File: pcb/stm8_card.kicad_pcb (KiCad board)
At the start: 2 copper layers, 101.9 x 50.9 mm, 22 parts, among them J1 DEBUG HEADER, SW1 TL59AF100Q, SW2 TL59AF100Q, SW3 TL59AF100Q, SW4 TL3302AF260QG, U1 ER-OLED0.91-7, U2 STM8S103F3

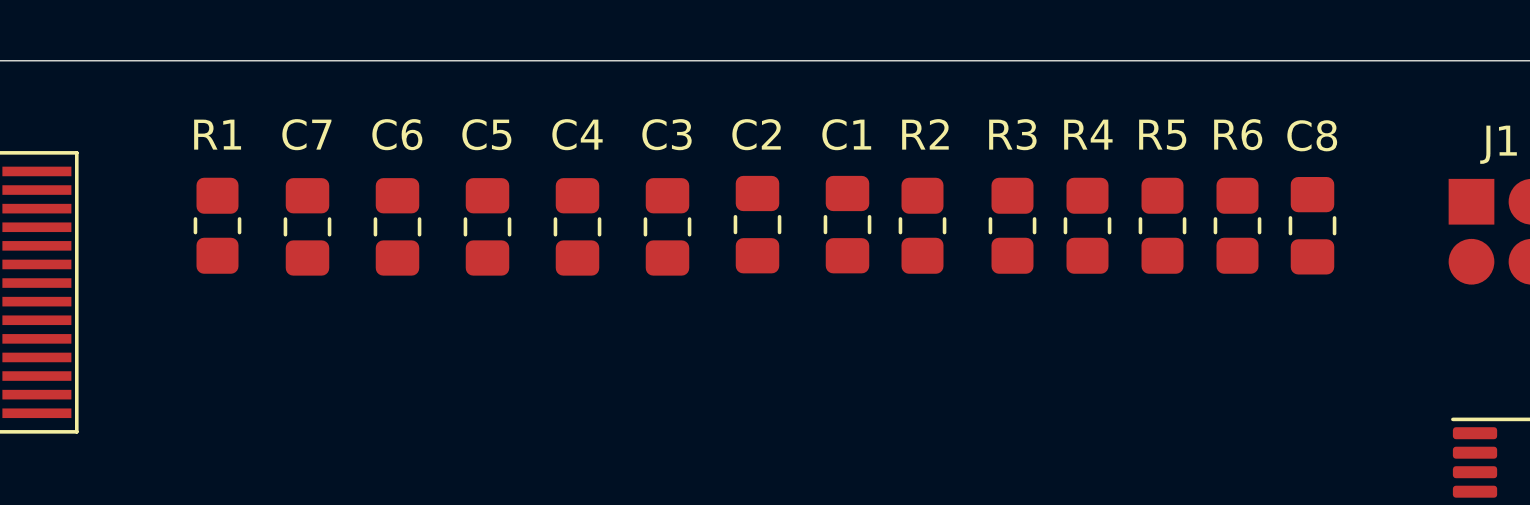
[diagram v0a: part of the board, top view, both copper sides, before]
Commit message: pcb small edits
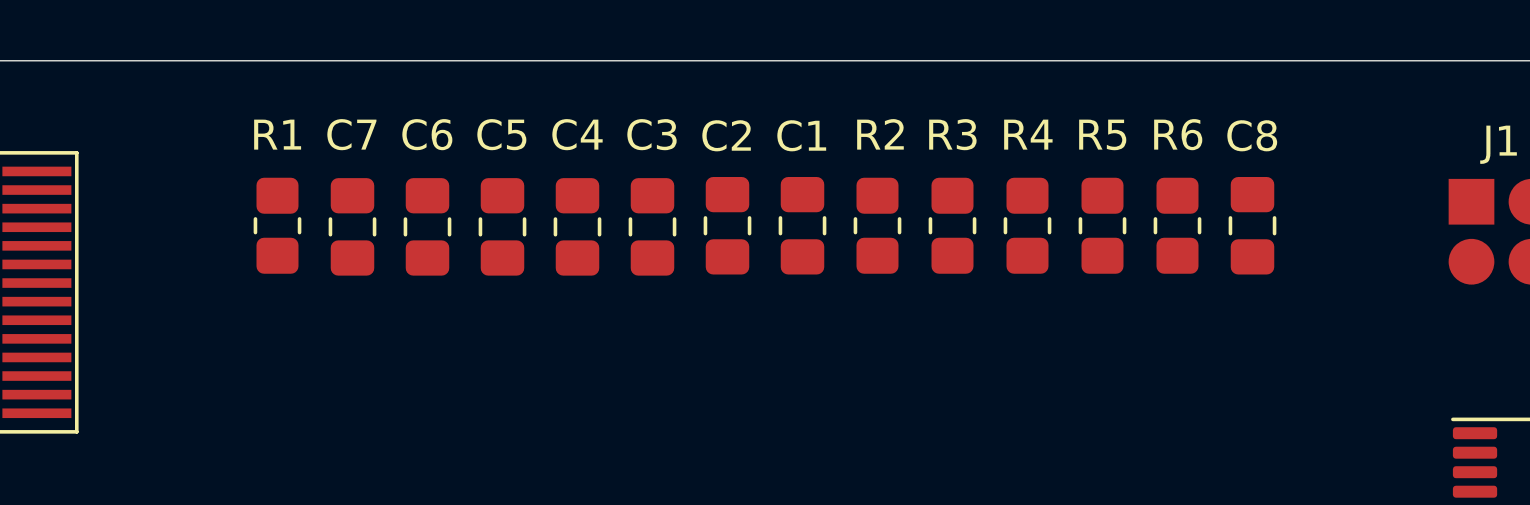
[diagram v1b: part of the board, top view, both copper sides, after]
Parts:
- moved C8 2.00 mm to (261.5, 107.0)
- moved R1 2.00 mm to (229.0, 107.0)
- moved R3 2.00 mm to (251.5, 107.0)
- moved R4 2.00 mm to (254.0, 107.0), turned to 270 degrees
- moved R5 2.00 mm to (256.5, 107.0)
- moved R6 2.00 mm to (259.0, 107.0)
- moved C1 1.50 mm to (246.5, 107.0)
- moved C7 1.50 mm to (231.5, 107.0)
- moved R2 1.50 mm to (249.0, 107.0)
- moved C2 1.00 mm to (244.0, 107.0)
- moved C6 1.00 mm to (234.0, 107.0)
- moved C3 0.50 mm to (241.5, 107.0)
- moved C5 0.50 mm to (236.5, 107.0)
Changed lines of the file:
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@@
   )
   (module Capacitor_SMD:C_0805_2012Metric_Pad1.18x1.45mm_HandSolder (layer F.Cu)
-    (at 248 106.9625 90)
+    (at 246.5 107 90)
     (descr "Capacitor SMD 0805 (2012 Metric), square (rectangular) end terminal, IPC_7351 nominal with elongated pad for handsoldering. (Body size source: IPC-SM-782 page 76, https://www.pcb-3d.com/wordpress/wp-content/uploads/ipc-sm-782a_amendment_1_and_2.pdf, https://docs.google.com/spreadsheets/d/1BsfQQcO9C6DZCsRaXUlFlo91Tg2WpOkGARC1WS5S8t0/edit?usp=sharing), generated with kicad-footprint-generator")
     (tags "capacitor handsolder")
@@
   )
   (module Capacitor_SMD:C_0805_2012Metric_Pad1.18x1.45mm_HandSolder (layer F.Cu)
-    (at 245 106.9625 90)
+    (at 244 107 90)
     (descr "Capacitor SMD 0805 (2012 Metric), square (rectangular) end terminal, IPC_7351 nominal with elongated pad for handsoldering. (Body size source: IPC-SM-782 page 76, https://www.pcb-3d.com/wordpress/wp-content/uploads/ipc-sm-782a_amendment_1_and_2.pdf, https://docs.google.com/spreadsheets/d/1BsfQQcO9C6DZCsRaXUlFlo91Tg2WpOkGARC1WS5S8t0/edit?usp=sharing), generated with kicad-footprint-generator")
     (tags "capacitor handsolder")
@@
   )
   (module Capacitor_SMD:C_0805_2012Metric_Pad1.18x1.45mm_HandSolder (layer F.Cu)
-    (at 242 107.0375 90)
+    (at 241.5 107.0375 90)
     (descr "Capacitor SMD 0805 (2012 Metric), square (rectangular) end terminal, IPC_7351 nominal with elongated pad for handsoldering. (Body size source: IPC-SM-782 page 76, https://www.pcb-3d.com/wordpress/wp-content/uploads/ipc-sm-782a_amendment_1_and_2.pdf, https://docs.google.com/spreadsheets/d/1BsfQQcO9C6DZCsRaXUlFlo91Tg2WpOkGARC1WS5S8t0/edit?usp=sharing), generated with kicad-footprint-generator")
     (tags "capacitor handsolder")
@@
   )
   (module Capacitor_SMD:C_0805_2012Metric_Pad1.18x1.45mm_HandSolder (layer F.Cu)
-    (at 236 107.0375 270)
+    (at 236.5 107.0375 270)
     (descr "Capacitor SMD 0805 (2012 Metric), square (rectangular) end terminal, IPC_7351 nominal with elongated pad for handsoldering. (Body size source: IPC-SM-782 page 76, https://www.pcb-3d.com/wordpress/wp-content/uploads/ipc-sm-782a_amendment_1_and_2.pdf, https://docs.google.com/spreadsheets/d/1BsfQQcO9C6DZCsRaXUlFlo91Tg2WpOkGARC1WS5S8t0/edit?usp=sharing), generated with kicad-footprint-generator")
     (tags "capacitor handsolder")
@@
   )
   (module Capacitor_SMD:C_0805_2012Metric_Pad1.18x1.45mm_HandSolder (layer F.Cu)
-    (at 233 107.0375 270)
+    (at 234 107.0375 270)
     (descr "Capacitor SMD 0805 (2012 Metric), square (rectangular) end terminal, IPC_7351 nominal with elongated pad for handsoldering. (Body size source: IPC-SM-782 page 76, https://www.pcb-3d.com/wordpress/wp-content/uploads/ipc-sm-782a_amendment_1_and_2.pdf, https://docs.google.com/spreadsheets/d/1BsfQQcO9C6DZCsRaXUlFlo91Tg2WpOkGARC1WS5S8t0/edit?usp=sharing), generated with kicad-footprint-generator")
     (tags "capacitor handsolder")
@@
   )
   (module Capacitor_SMD:C_0805_2012Metric_Pad1.18x1.45mm_HandSolder (layer F.Cu)
-    (at 230 107.0375 270)
+    (at 231.5 107.0375 270)
     (descr "Capacitor SMD 0805 (2012 Metric), square (rectangular) end terminal, IPC_7351 nominal with elongated pad for handsoldering. (Body size source: IPC-SM-782 page 76, https://www.pcb-3d.com/wordpress/wp-content/uploads/ipc-sm-782a_amendment_1_and_2.pdf, https://docs.google.com/spreadsheets/d/1BsfQQcO9C6DZCsRaXUlFlo91Tg2WpOkGARC1WS5S8t0/edit?usp=sharing), generated with kicad-footprint-generator")
     (tags "capacitor handsolder")
@@
   )
   (module Capacitor_SMD:C_0805_2012Metric_Pad1.18x1.45mm_HandSolder (layer F.Cu)
-    (at 263.5 107 90)
+    (at 261.5 107 90)
     (descr "Capacitor SMD 0805 (2012 Metric), square (rectangular) end terminal, IPC_7351 nominal with elongated pad for handsoldering. (Body size source: IPC-SM-782 page 76, https://www.pcb-3d.com/wordpress/wp-content/uploads/ipc-sm-782a_amendment_1_and_2.pdf, https://docs.google.com/spreadsheets/d/1BsfQQcO9C6DZCsRaXUlFlo91Tg2WpOkGARC1WS5S8t0/edit?usp=sharing), generated with kicad-footprint-generator")
     (tags "capacitor handsolder")
@@
   )
   (module Resistor_SMD:R_0805_2012Metric_Pad1.20x1.40mm_HandSolder (layer F.Cu)
-    (at 227 107 90)
+    (at 229 107 90)
     (descr "Resistor SMD 0805 (2012 Metric), square (rectangular) end terminal, IPC_7351 nominal with elongated pad for handsoldering. (Body size source: IPC-SM-782 page 72, https://www.pcb-3d.com/wordpress/wp-content/uploads/ipc-sm-782a_amendment_1_and_2.pdf), generated with kicad-footprint-generator")
     (tags "resistor handsolder")
@@
   )
   (module Resistor_SMD:R_0805_2012Metric_Pad1.20x1.40mm_HandSolder (layer F.Cu)
-    (at 250.5 107 90)
+    (at 249 107 90)
     (descr "Resistor SMD 0805 (2012 Metric), square (rectangular) end terminal, IPC_7351 nominal with elongated pad for handsoldering. (Body size source: IPC-SM-782 page 72, https://www.pcb-3d.com/wordpress/wp-content/uploads/ipc-sm-782a_amendment_1_and_2.pdf), generated with kicad-footprint-generator")
     (tags "resistor handsolder")
@@
   )
   (module Resistor_SMD:R_0805_2012Metric_Pad1.20x1.40mm_HandSolder (layer F.Cu)
-    (at 253.5 107 90)
+    (at 251.5 107 90)
     (descr "Resistor SMD 0805 (2012 Metric), square (rectangular) end terminal, IPC_7351 nominal with elongated pad for handsoldering. (Body size source: IPC-SM-782 page 72, https://www.pcb-3d.com/wordpress/wp-content/uploads/ipc-sm-782a_amendment_1_and_2.pdf), generated with kicad-footprint-generator")
     (tags "resistor handsolder")
@@
   )
   (module Resistor_SMD:R_0805_2012Metric_Pad1.20x1.40mm_HandSolder (layer F.Cu)
-    (at 256 107 90)
-    (descr "Resistor SMD 0805 (2012 Metric), square (rectangular) end terminal, IPC_7351 nominal with elongated pad for handsoldering. (Body size source: IPC-SM-782 page 72, https://www.pcb-3d.com/wordpress/wp-content/uploads/ipc-sm-782a_amendment_1_and_2.pdf), generated with kicad-footprint-generator")
-    (tags "resistor handsolder")
-    (attr smd)
-    (fp_text reference R4 (at 3 0 180) (layer F.SilkS)
+    (at 254 107 270)
+    (descr "Resistor SMD 0805 (2012 Metric), square (rectangular) end terminal, IPC_7351 nominal with elongated pad for handsoldering. (Body size source: IPC-SM-782 page 72, https://www.pcb-3d.com/wordpress/wp-content/uploads/ipc-sm-782a_amendment_1_and_2.pdf), generated with kicad-footprint-generator")
+    (tags "resistor handsolder")
+    (attr smd)
+    (fp_text reference R4 (at -3 0 180) (layer F.SilkS)
       (effects (font (size 1 1) (thickness 0.15)))
     )
@@
       (effects (font (size 0.5 0.5) (thickness 0.08)))
     )
-    (pad 1 smd roundrect (at -1 0 90) (size 1.2 1.4) (layers F.Cu F.Paste F.Mask) (roundrect_rratio 0.208333)
-      (net 1 GND))
-    (pad 2 smd roundrect (at 1 0 90) (size 1.2 1.4) (layers F.Cu F.Paste F.Mask) (roundrect_rratio 0.208333)
+    (pad 1 smd roundrect (at -1 0 270) (size 1.2 1.4) (layers F.Cu F.Paste F.Mask) (roundrect_rratio 0.208333)
+      (net 1 GND))
+    (pad 2 smd roundrect (at 1 0 270) (size 1.2 1.4) (layers F.Cu F.Paste F.Mask) (roundrect_rratio 0.208333)
       (net 20 btn0))
     (model ${KISYS3DMOD}/Resistor_SMD.3dshapes/R_0805_2012Metric.wrl
@@
   )
   (module Resistor_SMD:R_0805_2012Metric_Pad1.20x1.40mm_HandSolder (layer F.Cu)
-    (at 258.5 107 270)
+    (at 256.5 107 270)
     (descr "Resistor SMD 0805 (2012 Metric), square (rectangular) end terminal, IPC_7351 nominal with elongated pad for handsoldering. (Body size source: IPC-SM-782 page 72, https://www.pcb-3d.com/wordpress/wp-content/uploads/ipc-sm-782a_amendment_1_and_2.pdf), generated with kicad-footprint-generator")
     (tags "resistor handsolder")
@@
   )
   (module Resistor_SMD:R_0805_2012Metric_Pad1.20x1.40mm_HandSolder (layer F.Cu)
-    (at 261 107 270)
-    (descr "Resistor SMD 0805 (2012 Metric), square (rectangular) end terminal, IPC_7351 nominal with elongated pad for handsoldering. (Body size source: IPC-SM-782 page 72, https://www.pcb-3d.com/wordpress/wp-content/uploads/ipc-sm-782a_amendment_1_and_2.pdf), generated with kicad-footprint-generator")
-    (tags "resistor handsolder")
+    (at 259 107 270)
+    (descr "Resistor SMD 0805 (2012 Metric), square (rectangular) end terminal, IPC_7351 nominal with elongated pad for handsoldering. (Body size source: IPC-SM-782 page 72, https://www.pcb-3d.com/wordpress/wp-content/uploads/ipc-sm-782a_amendment_1_and_2.pdf), generated with kicad-footprint-generator")
+    (tags "resistor handsolder")

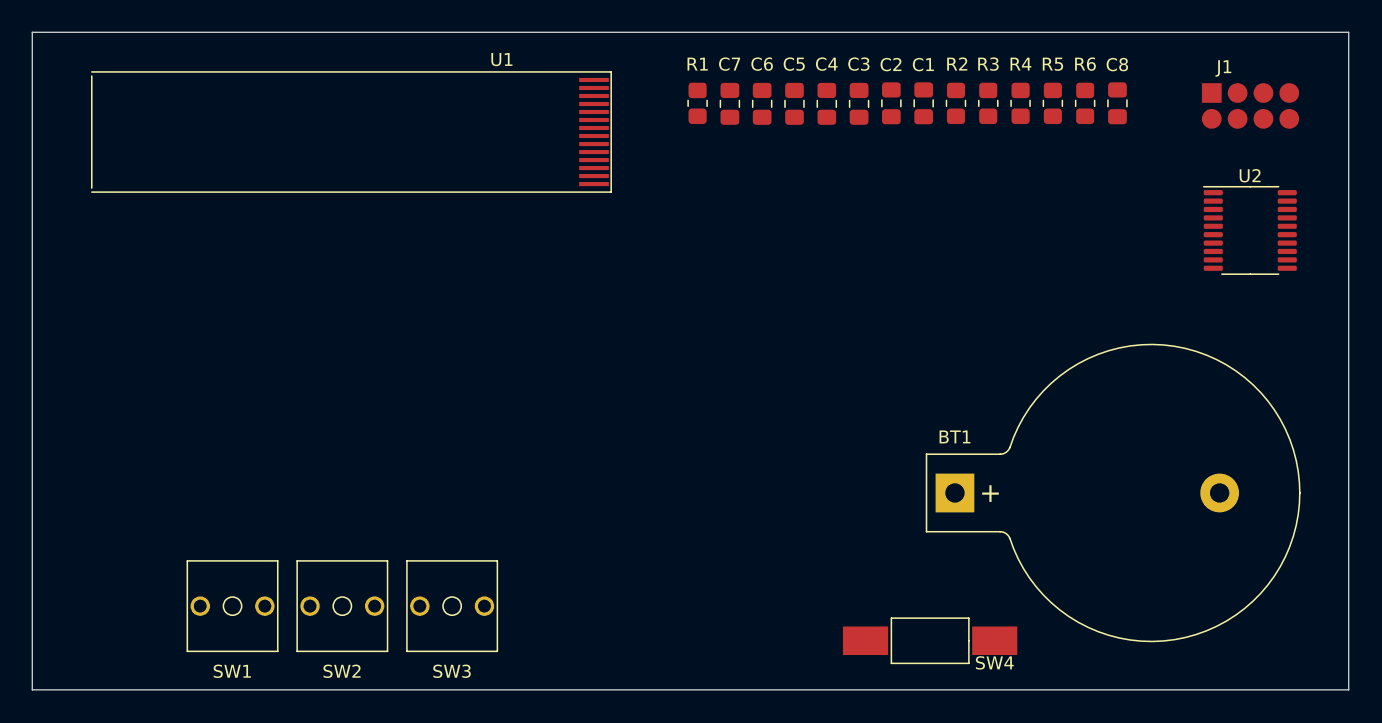
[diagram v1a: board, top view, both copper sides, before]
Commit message: pcb technically finished I think?
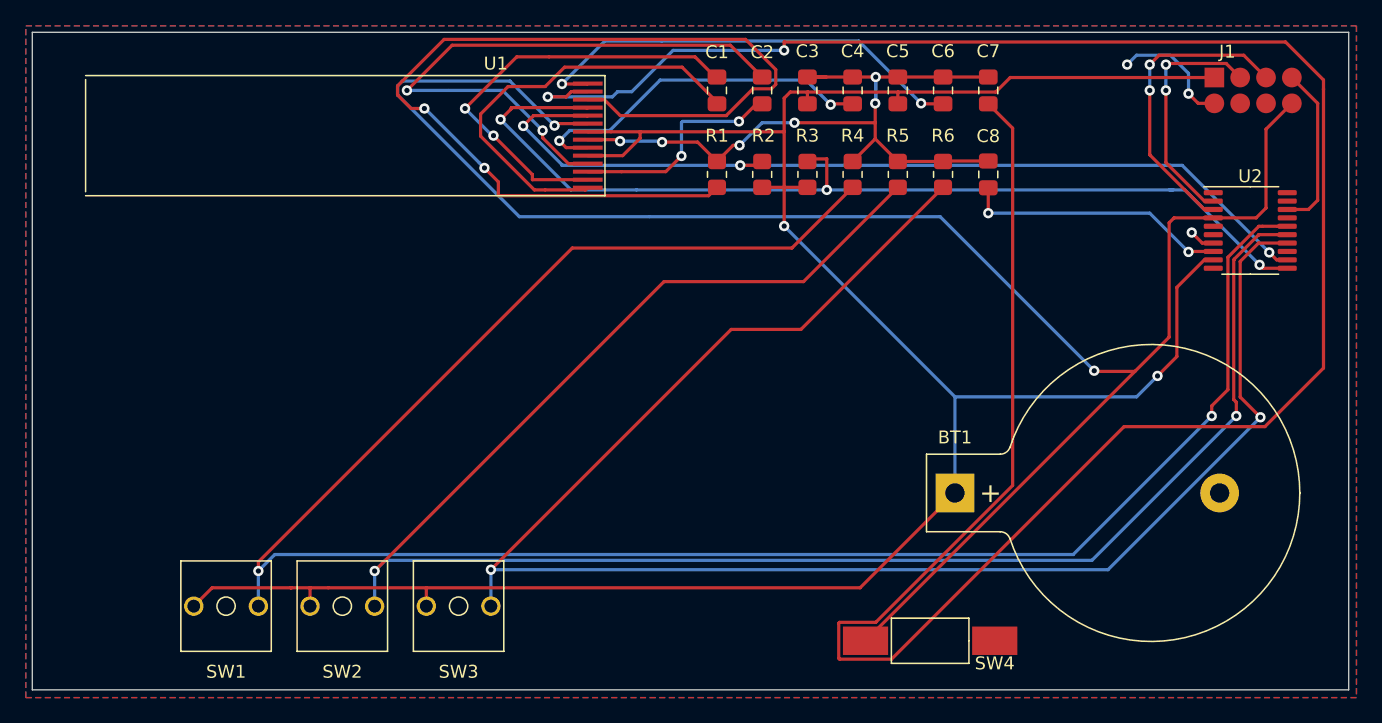
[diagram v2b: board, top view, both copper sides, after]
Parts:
- moved C7 20.0 mm to (251.5, 106.0)
- moved C1 16.0 mm to (230.5, 106.0)
- moved R2 16.0 mm to (234.0, 112.5)
- moved R3 15.0 mm to (237.5, 112.5)
- moved R4 14.1 mm to (241.0, 112.5)
- moved C6 14.0 mm to (248.0, 106.0)
- moved R5 13.2 mm to (244.5, 112.5)
- moved R6 12.3 mm to (248.0, 112.5)
- moved C8 11.4 mm to (251.5, 112.5)
- moved C2 10.0 mm to (234.0, 106.0)
- moved C5 8.07 mm to (244.5, 106.0)
- moved R1 5.70 mm to (230.5, 112.5)
- moved C3 4.13 mm to (237.5, 106.0)
- moved C4 2.25 mm to (241.0, 106.0)
- moved J1 1.22 mm to (272.0, 106.0)
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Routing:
- net 3v3: track 0.00 -> 188.7 mm, vias 0 -> 2
- net Net-(C7-Pad2): track 0.00 -> 186.9 mm, vias 0 -> 2
- net btn0: track 0.00 -> 159.3 mm, vias 0 -> 2
- net btn1: track 0.00 -> 145.0 mm, vias 0 -> 2
- net NRST: track 0.00 -> 142.7 mm, vias 0 -> 2
- net btn2: track 0.00 -> 131.5 mm, vias 0 -> 2
- net Net-(R1-Pad1): track 0.00 -> 78.5 mm, vias 0 -> 2
- net SDA: track 0.00 -> 77.2 mm, vias 0 -> 3
- net SCL: track 0.00 -> 71.0 mm, vias 0 -> 3
- net GND: track 0.00 -> 69.8 mm, vias 0 -> 9
- net Net-(C2-Pad2): track 0.00 -> 48.3 mm, vias 0 -> 2
- net Net-(C6-Pad2): track 0.00 -> 34.9 mm, vias 0 -> 2
- net Net-(C1-Pad2): track 0.00 -> 33.8 mm, vias 0 -> 2
- net Net-(C1-Pad1): track 0.00 -> 32.9 mm
- net Net-(C4-Pad1): track 0.00 -> 27.9 mm, vias 0 -> 2
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- added copper zone on B.Cu, net GND
- added copper zone on F.Cu, net GND
